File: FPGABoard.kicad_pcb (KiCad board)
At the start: 2 copper layers, 100 x 80 mm, 86 parts, among them P1 JTAG_FPGA, P2 CONN_02X03, P3 USB_B, P4 CONN_02X07, P5 JTAG, P6 CONN_02X07, P7 CONN_02X07, P8 CONN_02X07, Q1 Q_NMOS_DSG, SW1 SW_PUSH, SW2 SW_PUSH, U1 XC3S50A/VQ100, U2 LM317_SOT223, U3 LM317_SOT223, U4 LM317_SOT223, U5 ATMEGA32U4RC-A, U6 M25P20, U7 XO53, Y1 12MHz

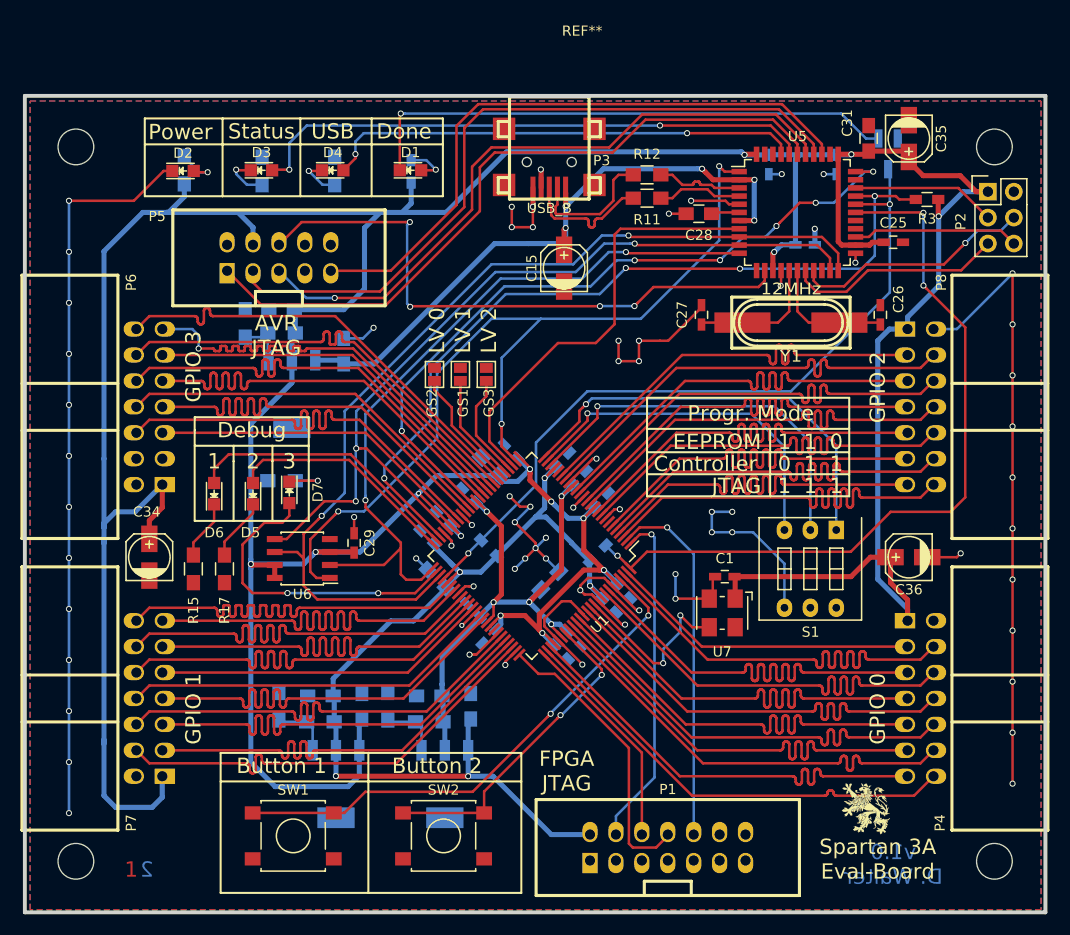
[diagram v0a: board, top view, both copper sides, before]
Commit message: Small update
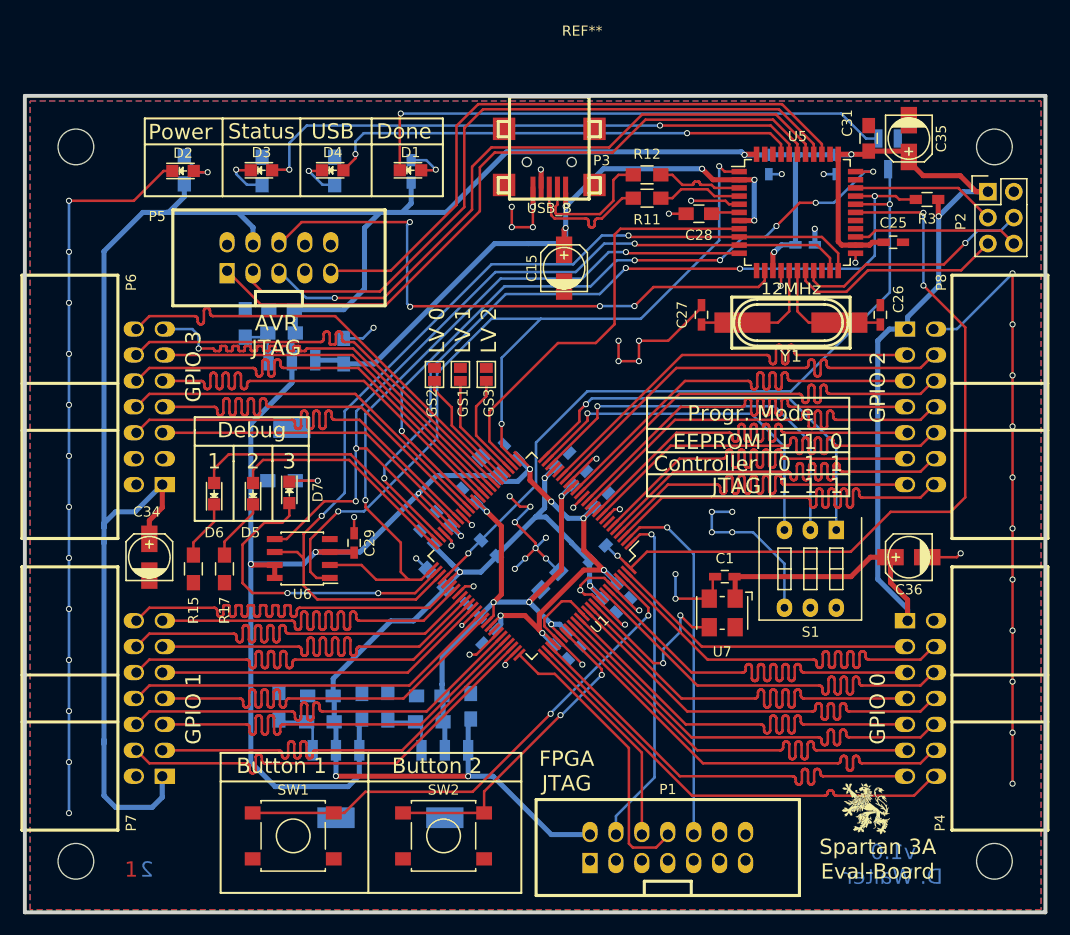
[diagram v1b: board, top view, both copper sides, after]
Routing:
- net /Microcontroller/MISO: track 71.9 -> 72.4 mm
